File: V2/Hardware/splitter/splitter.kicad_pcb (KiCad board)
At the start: 2 copper layers, 19 parts, among them J0 Rpi_40Pin_F, J1 Control_seg:1, J2 Control_seg:2, J3 Control_seg:3, J4 Molex_PSU_F, J5 Siren, J6 USB_A_F, K0 RELRAS0515, Q0 BC548C, Q1 BD139-16

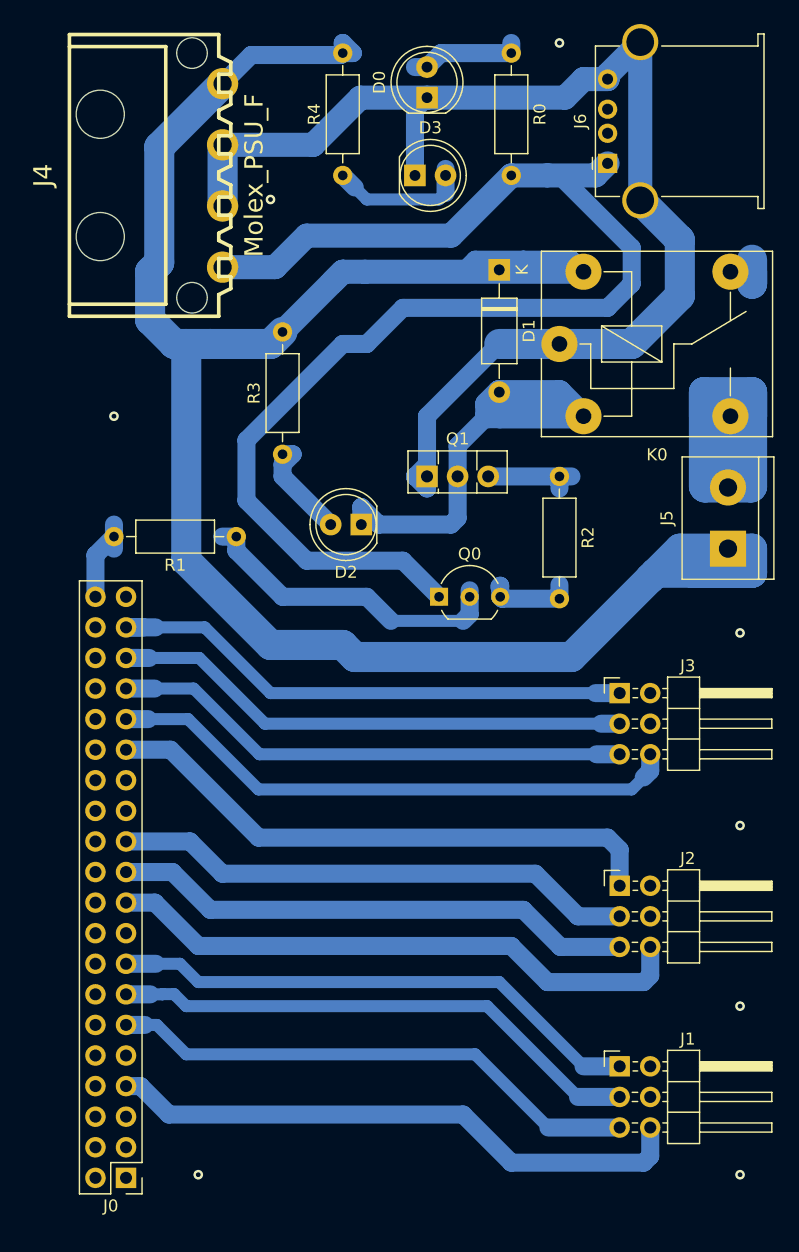
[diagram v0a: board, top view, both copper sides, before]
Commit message: Update splitter board
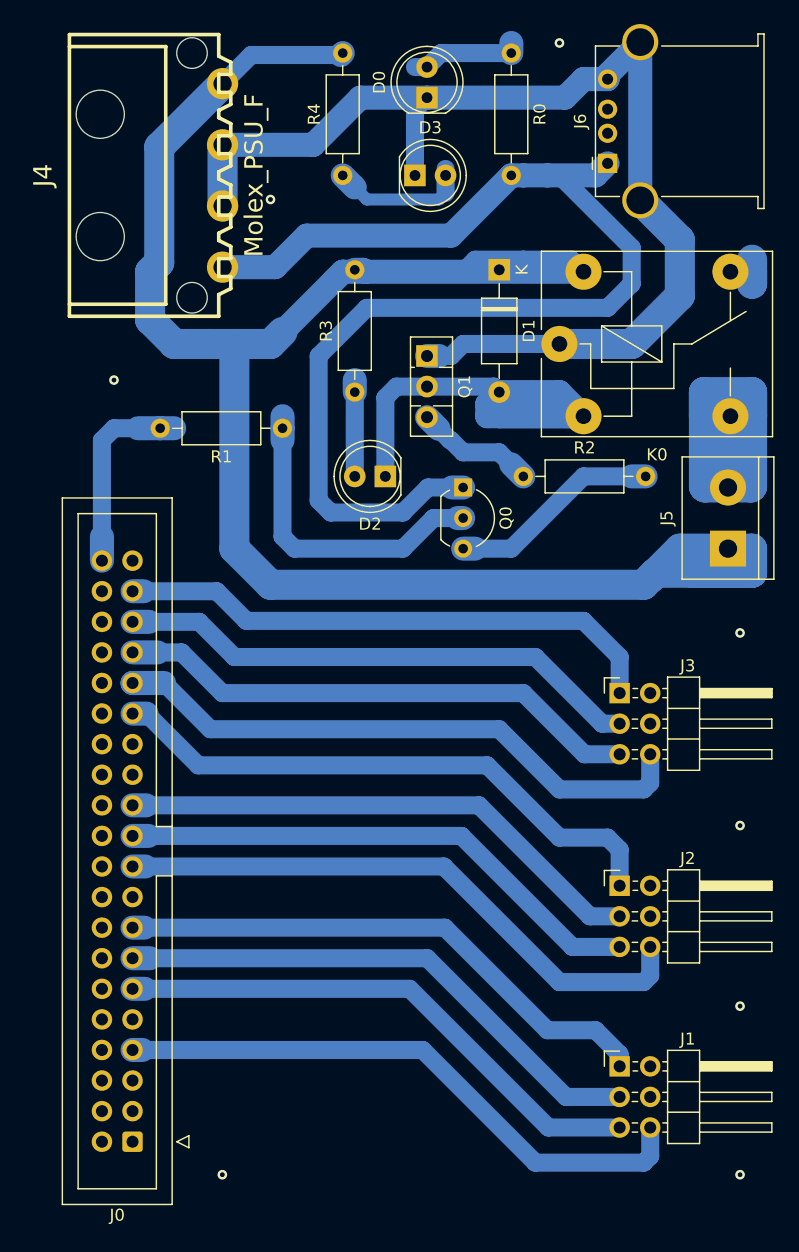
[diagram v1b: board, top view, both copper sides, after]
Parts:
- J0: footprint Connector_PinHeader_2.54mm:PinHeader_2x20_P2.54mm_Vertical -> Connector_IDC:IDC-Header_2x20_P2.54mm_Vertical
- moved Q1 10.0 mm to (149.0, 67.0), turned to 270 degrees
- moved R1 9.78 mm to (137.0, 73.0)
- moved Q0 9.30 mm to (152.0, 77.9), turned to 270 degrees
- moved R3 7.91 mm to (143.0, 70.0)
- moved D2 4.47 mm to (145.5, 77.0)
- moved J0 3.05 mm to (124.5, 132.3)
- moved R2 3.00 mm to (157.0, 77.0), turned to 0 degrees
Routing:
- net Earth: track 107.8 -> 95.9 mm
- net /12V+: track 188.7 -> 177.9 mm
- net Net-(Q0-Pad3): track 7.18 -> 17.6 mm
- net /SIREN_gpio:21: track 7.64 -> 16.4 mm
- net /5V+: track 109.7 -> 101.8 mm
- net /seg:3_bit:a_gpio:06: track 48.0 -> 51.9 mm
- net Net-(D1-Pad2): track 48.0 -> 44.8 mm
- net Net-(Q1-Pad3): track 7.92 -> 10.0 mm
- net /seg:3_bit:c_gpio:19: track 45.3 -> 44.0 mm
- net /seg:1_bit:d_gpio:22: track 44.5 -> 45.8 mm
- net /seg:3_bit:b_gpio:13: track 43.3 -> 44.0 mm
- net /seg:2_bit:c_gpio:11: track 43.6 -> 44.3 mm
- net /seg:2_bit:a_gpio:10: track 48.9 -> 49.6 mm
- net /seg:2_bit:b_gpio:09: track 43.6 -> 44.3 mm
- net /seg:1_bit:b_gpio:17: track 44.5 -> 45.2 mm
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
